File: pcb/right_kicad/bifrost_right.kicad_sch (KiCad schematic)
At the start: 64 parts, among them J1 HRO_TYPE-C-31-M-12, J2 Conn_01x02, J3 Conn_01x06, J4 Conn_01x05, Q1 AO3401A, Q2 2N7002, Q3 AO3401A, SW1 1U, SW10 1U, SW11 1U, SW12 1U, SW13 1U, SW14 1U, SW15 1U, SW16 1U, SW17 1U, SW18 2.25U, SW19 1U, SW2 1U, SW20 1U, SW21 1.5U, SW22 1U, SW23 1U, SW3 1U, SW4 1U, SW5 1U, SW6 1U, SW7 1U, SW8 1U, SW9 1U, T1 TS24CA, U1 MDBT50Q-1MV2, U2 TP4057, U3 SRV05-4, X1 32.768kHz

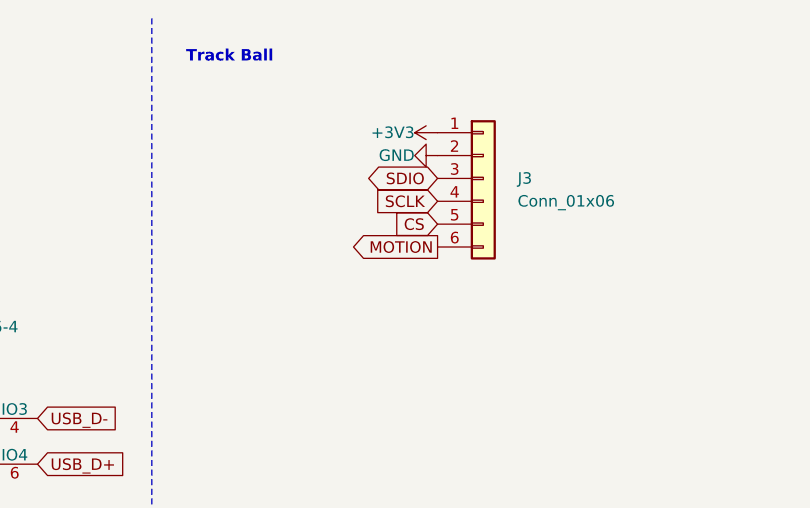
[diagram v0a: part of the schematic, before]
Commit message: Update PCB designs
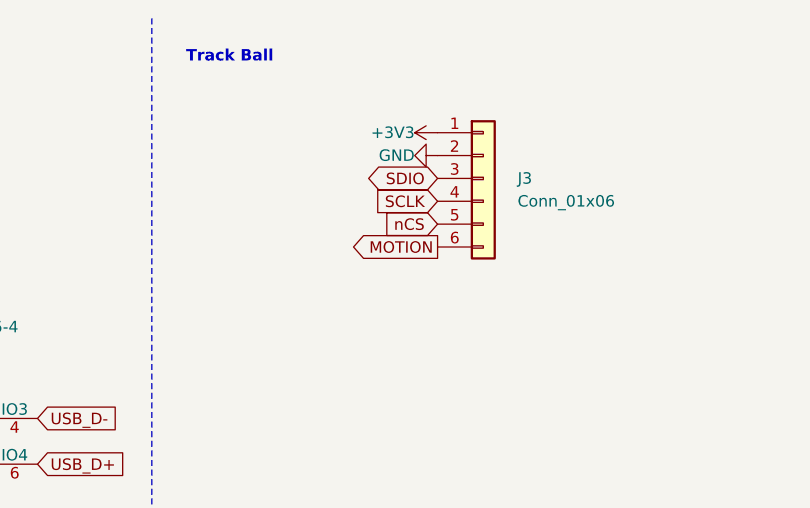
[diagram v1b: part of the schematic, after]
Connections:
- net CS: no longer J3.5 (Pin_5)
- new net nCS: J3.5 (Pin_5)
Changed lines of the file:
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@@
 		)
 	)
-	(global_label "CS"
+	(global_label "nCS"
 		(shape input)
 		(at 254 35.56 180)
@@
 		)
 		(property "Intersheetrefs" "${INTERSHEET_REFS}"
-			(at 248.5353 35.56 0)
+			(at 247.3863 35.56 0)
 			(hide yes)
 			(show_name no)
